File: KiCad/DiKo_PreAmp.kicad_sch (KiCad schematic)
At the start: 17 parts, among them J1 VCC_IN, J2 VCC_OUT, SW1 SW_DPST, U1 REC10K

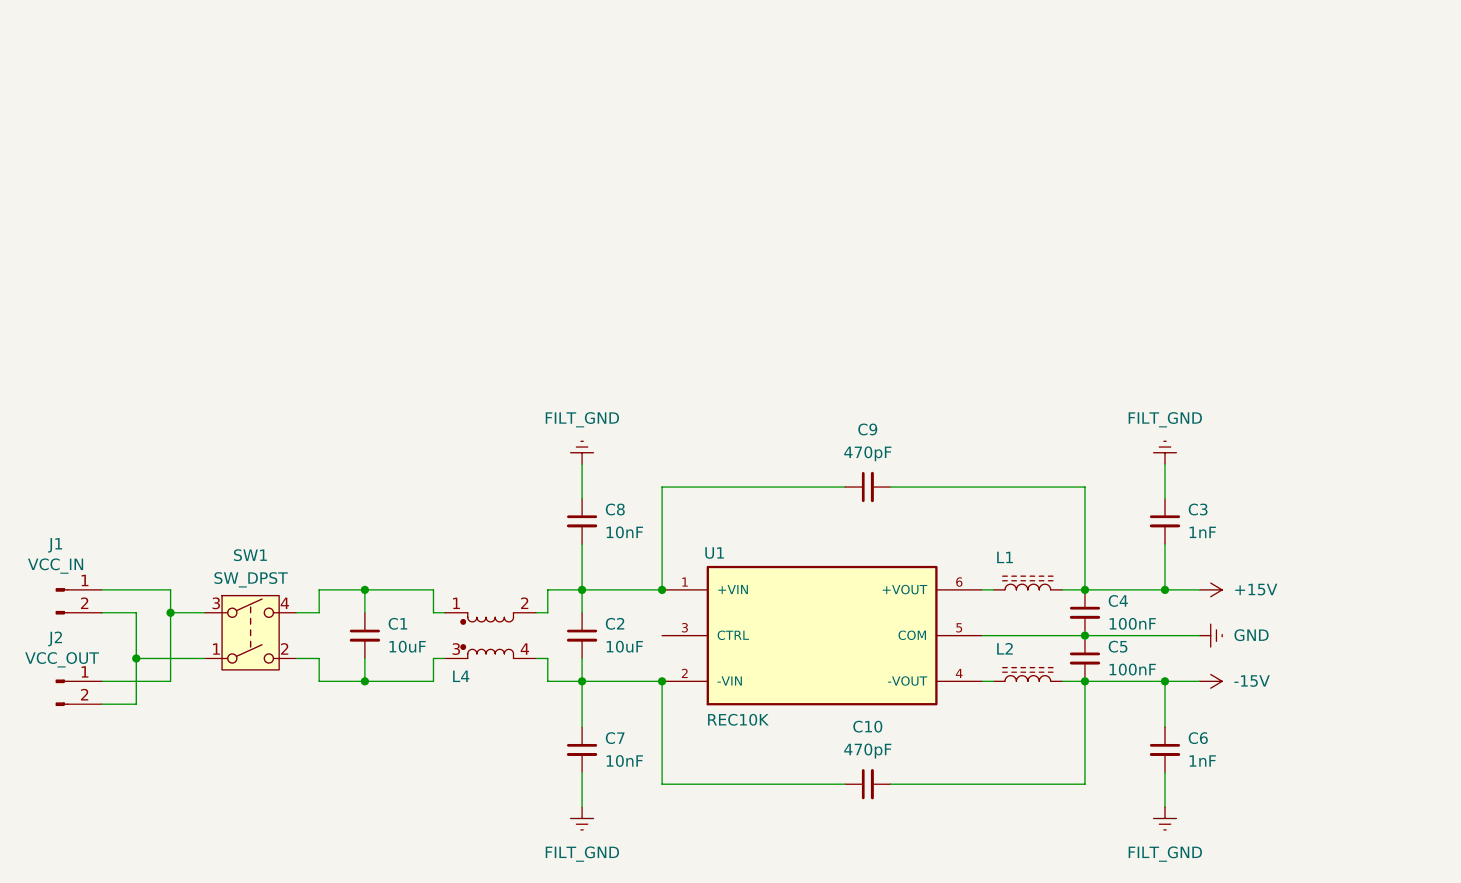
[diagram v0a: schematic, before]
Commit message: KiCad
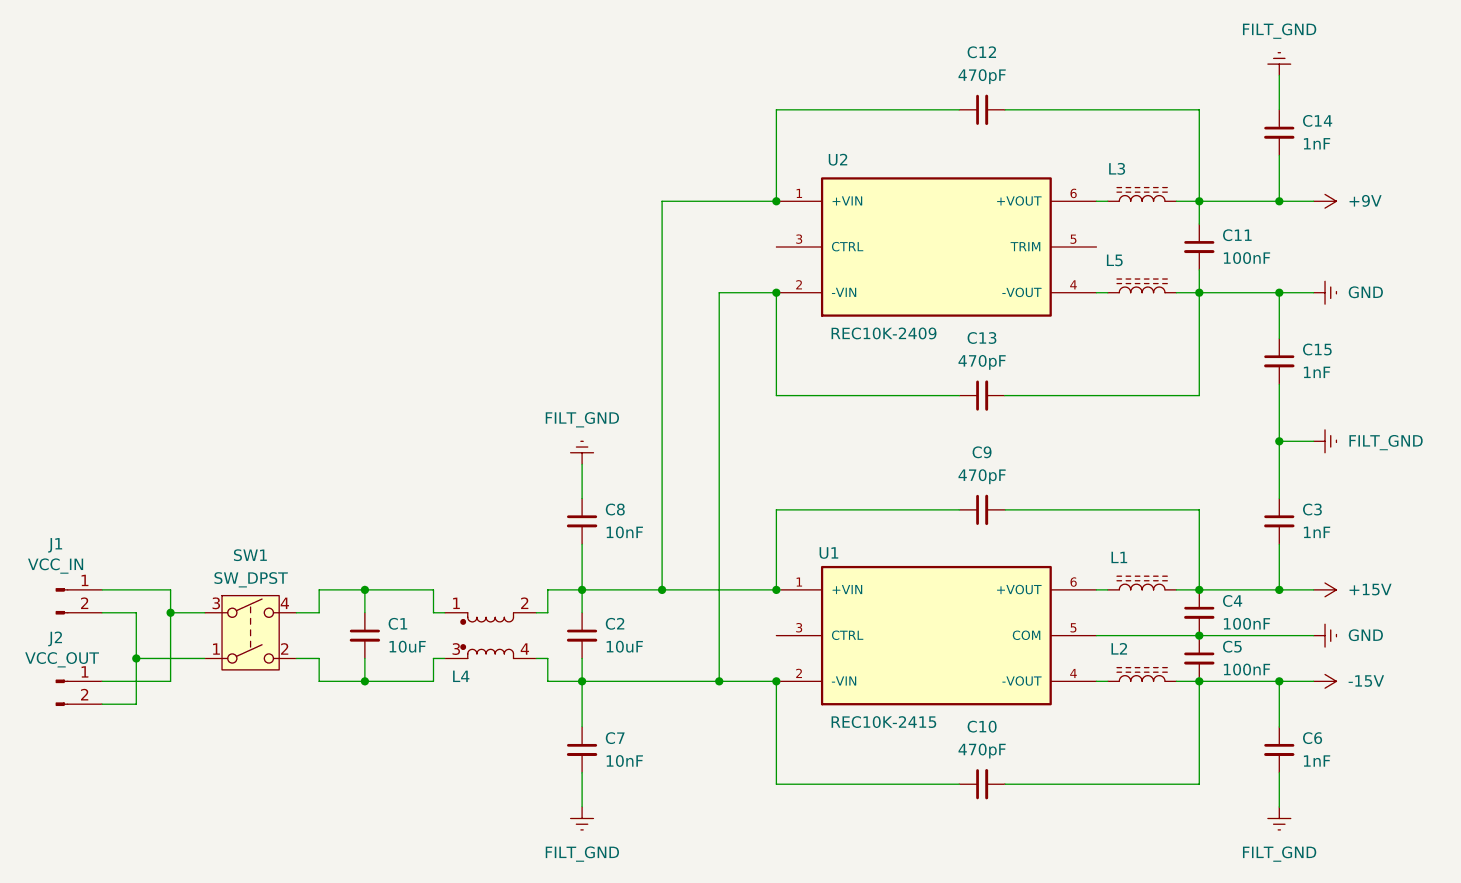
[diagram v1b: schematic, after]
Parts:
- added C11: 100nF, symbol Device:C_Small
- added C12, C13: 470pF, symbol Device:C_Small
- added C14, C15: 1nF, symbol Device:C_Small
- added L3: L_Ferrite, symbol Device:L_Ferrite
- added L5: ~, symbol Device:L_Ferrite
- added U2: REC10K-2409, REC10K-2409SAW_H2:CONV_REC10K-2409SAW_H2, symbol REC10K-2409SAW_H2:REC10K-2409SAW_H2
- U1: value REC10K -> REC10K-2415
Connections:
- net FILT_GND: now also C14.1, C15.2
- net GND: now also C11.2, C13.2, C15.1, L5.2
- net at C2.1, C8.2, C9.1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: now also C12.1, U2.1 (+VIN)
- net at C10.1, C2.2, C7.1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: now also C13.1, U2.2 (-VIN)
- new net: L5.1, U2.4 (-VOUT)
- new net: L3.1, U2.6 (+VOUT)
- new net +9V: C11.1, C12.2, C14.2, L3.2
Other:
- moved on the sheet: C10, C3, C4, C5, C6, C9, L1, L2, U1
